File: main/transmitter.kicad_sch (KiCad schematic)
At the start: 35 parts, among them Q1 PZT2222A, Q2 BS170, Q3 BS170, Q4 BS170, Q5 BS170, Q6 MMBT3904, Q7 BSS84, Q8 BS170, Q9 MMBT3904

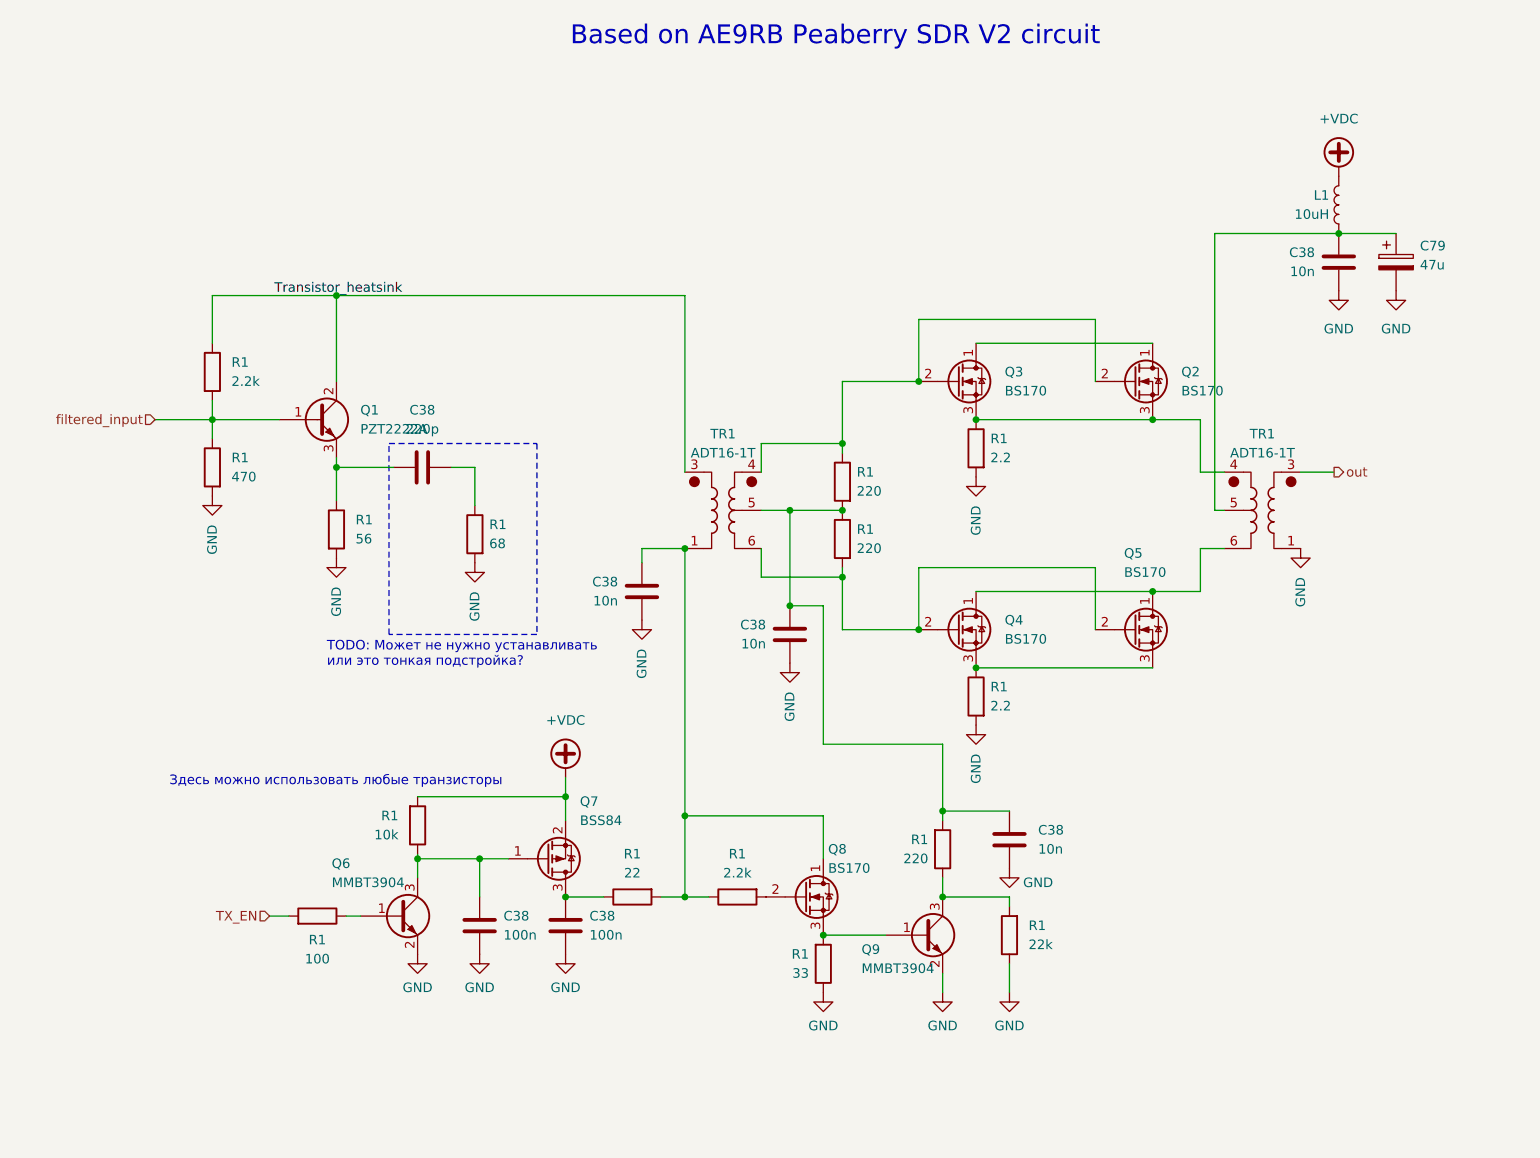
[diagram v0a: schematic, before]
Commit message: Power amplifier redraw
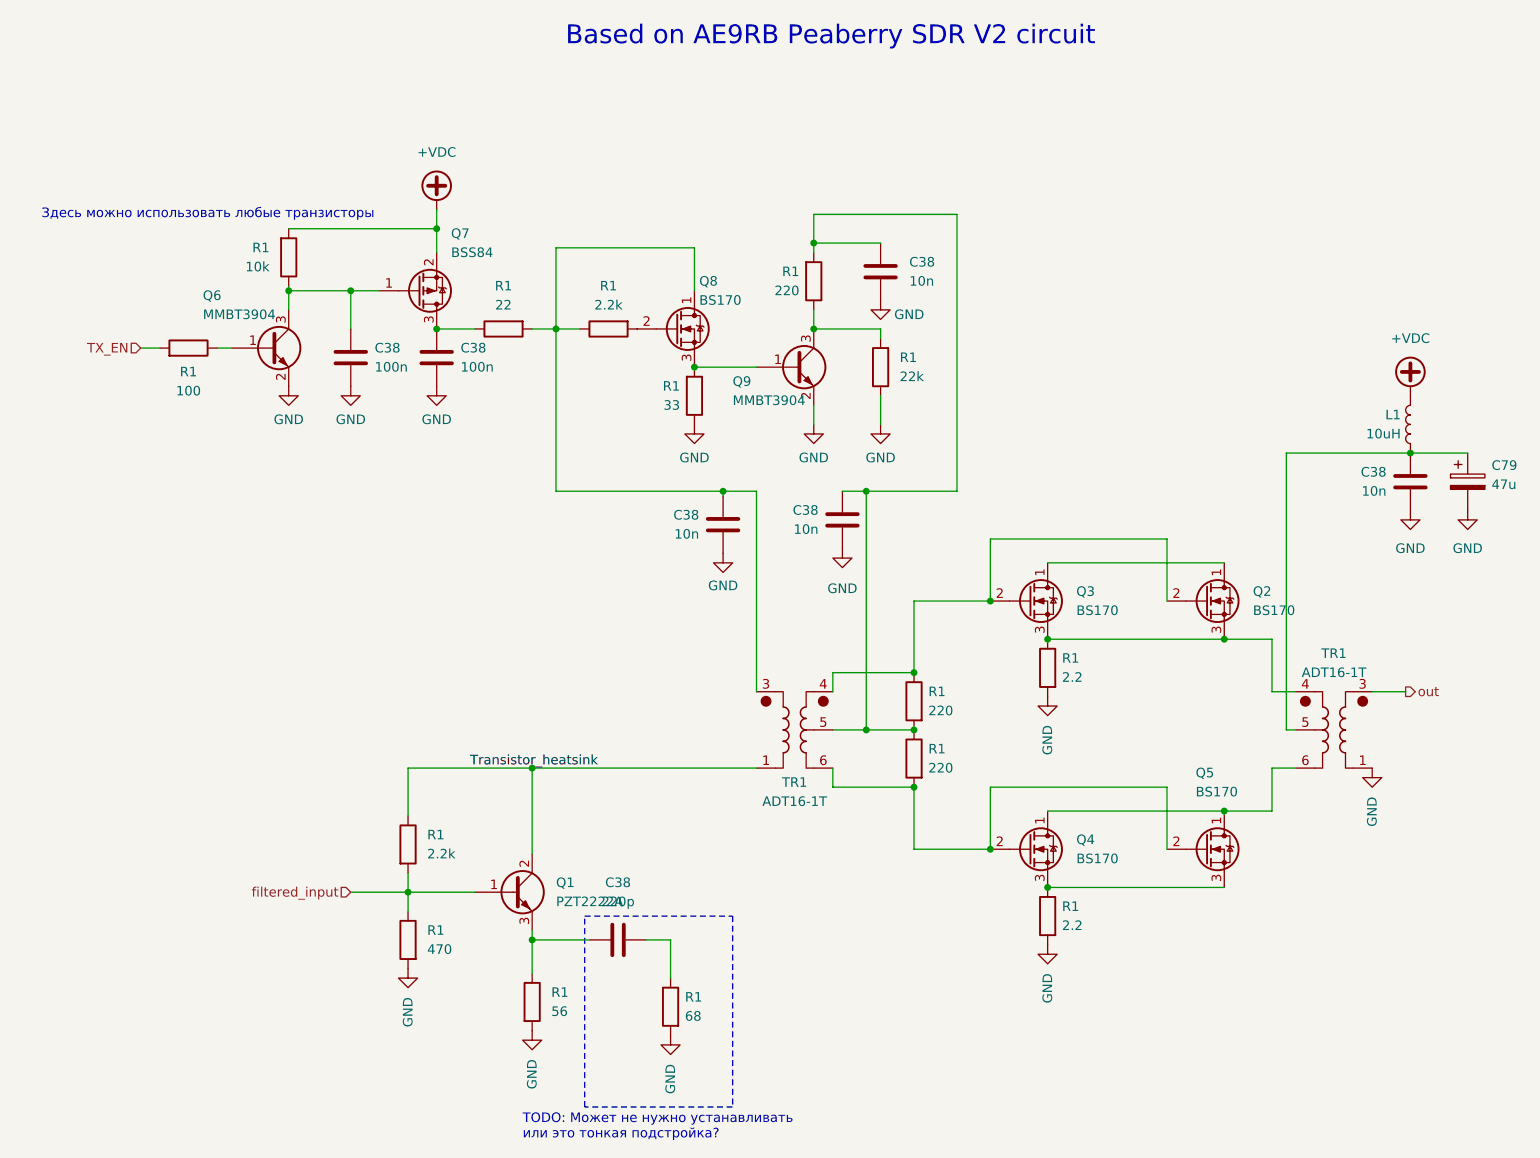
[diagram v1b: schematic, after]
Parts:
- removed C38 (x2): 100n, symbol Device:C
- removed C38: 10n, symbol Device:C
- removed R1: 2.2k, symbol Device:R
- removed R1: 10k, symbol Device:R
- removed R1: 22k, symbol Device:R
- removed R1: 33, symbol Device:R
- removed R1: 100, symbol Device:R
- removed R1: 220, symbol Device:R
- removed R1: 22, symbol Device:R
- added C38 (x2): 100n, symbol Device:C
- added C38: 10n, symbol Device:C
- added R1: 10k, symbol Device:R
- added R1: 33, symbol Device:R
- added R1: 100, symbol Device:R
- added R1: 220, symbol Device:R
- added R1: 22, symbol Device:R
- added R1: 22k, symbol Device:R
- added R1: 2.2k, symbol Device:R
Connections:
- net +VDC: now also R1.2
- net GND: now also C38.1, C38.1, C38.1, R1.1, R1.1
- net TX_EN: now also R1.2
- net Transistor_heatsink: now also TR1.1; no longer TR1.3
- net at C38.2, Q8.1 (D): now also TR1.3, R1.1, R1.2; no longer TR1.1
- net at Q8.2 (G): now also R1.2
- net at Q6.3 (C), Q7.1 (G): now also C38.2, R1.1
- net at Q9.3 (C): now also R1.1, R1.2
- net at Q8.3 (S), Q9.1 (B): now also R1.2
- net at Q6.1 (B): now also R1.1
- net at Q7.3 (D): now also C38.2, R1.1
- net at C38.2, R1.1, R1.2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: now also C38.2, R1.2
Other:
- moved on the sheet: C38, C79, L1, Q1, Q2, Q3, Q4, Q5, R1, TR1

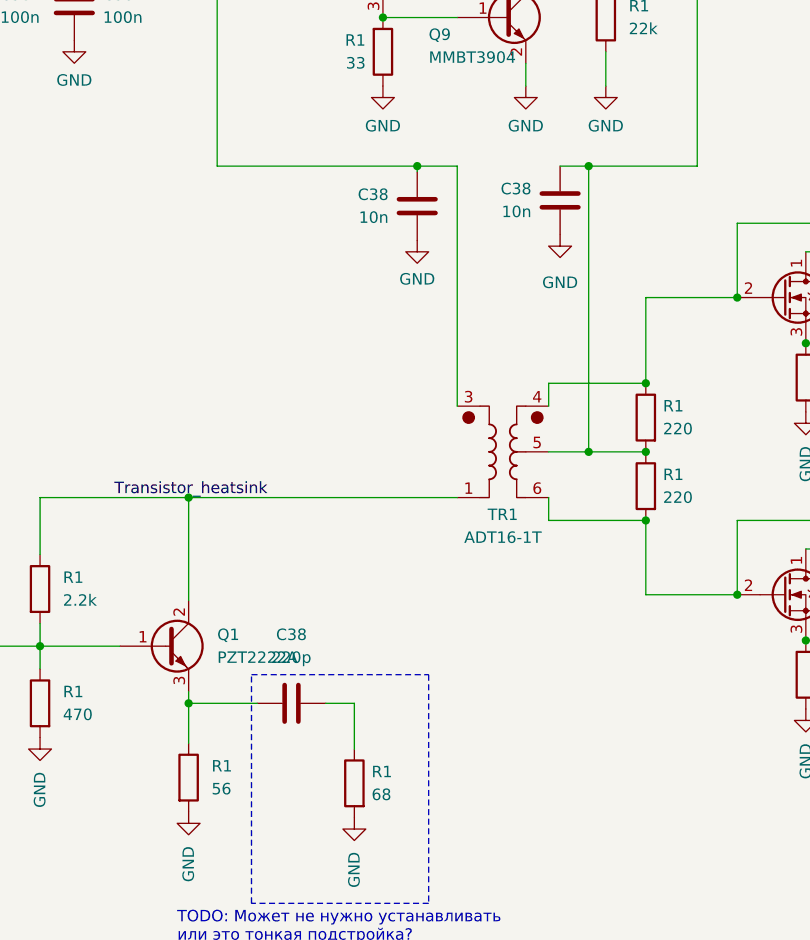
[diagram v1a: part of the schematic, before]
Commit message: 30 MHz output LPF added
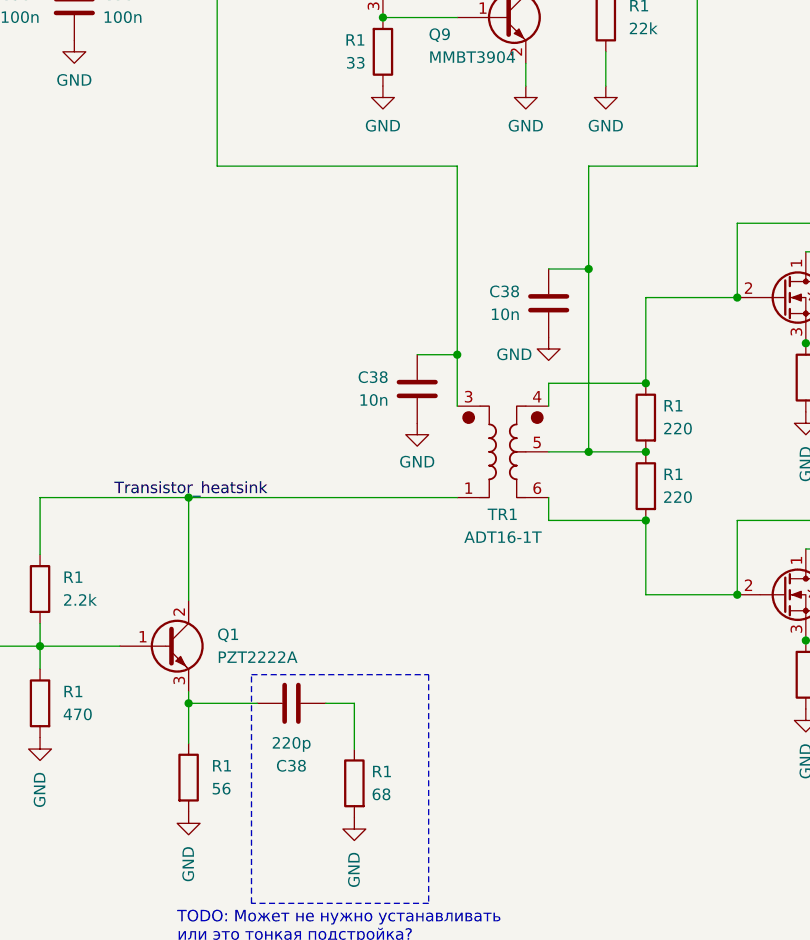
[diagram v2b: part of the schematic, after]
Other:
- moved on the sheet: C38
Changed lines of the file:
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@@
   (junction (at 147.955 112.395) (diameter 0) (color 0 0 0 0)
   )
+  (junction (at 147.955 92.075) (diameter 0) (color 0 0 0 0)
+  )
   (junction (at 90.805 45.72) (diameter 0) (color 0 0 0 0)
   )
@@
   (junction (at 154.305 112.395) (diameter 0) (color 0 0 0 0)
   )
-  (junction (at 147.955 80.645) (diameter 0) (color 0 0 0 0)
-  )
   (junction (at 140.97 47.625) (diameter 0) (color 0 0 0 0)
   )
@@
   (junction (at 172.085 100.33) (diameter 0) (color 0 0 0 0)
   )
-  (junction (at 128.905 80.645) (diameter 0) (color 0 0 0 0)
-  )
   (junction (at 71.12 53.975) (diameter 0) (color 0 0 0 0)
   )
@@
   (junction (at 195.58 100.33) (diameter 0) (color 0 0 0 0)
   )
+  (junction (at 133.35 101.6) (diameter 0) (color 0 0 0 0)
+  )
   (junction (at 164.465 128.27) (diameter 0) (color 0 0 0 0)
   )
@@
     (stroke (width 0) (type default))
   )
+  (wire (pts (xy 147.955 80.645) (xy 147.955 92.075))
+    (stroke (width 0) (type default))
+  )
   (wire (pts (xy 71.12 53.975) (xy 79.375 53.975))
     (stroke (width 0) (type default))
@@
     (stroke (width 0) (type default))
   )
-  (wire (pts (xy 147.955 80.645) (xy 147.955 112.395))
-    (stroke (width 0) (type default))
-  )
   (wire (pts (xy 140.97 56.515) (xy 140.97 59.055))
     (stroke (width 0) (type default))
@@
     (stroke (width 0) (type default))
   )
-  (wire (pts (xy 133.35 80.645) (xy 133.35 107.315))
+  (wire (pts (xy 133.35 80.645) (xy 133.35 101.6))
     (stroke (width 0) (type default))
   )
@@
     (stroke (width 0) (type default))
   )
-  (wire (pts (xy 106.68 80.645) (xy 128.905 80.645))
-    (stroke (width 0) (type default))
-  )
   (wire (pts (xy 51.435 61.595) (xy 53.975 61.595))
     (stroke (width 0) (type default))
@@
     (stroke (width 0) (type default))
   )
-  (wire (pts (xy 128.905 80.645) (xy 133.35 80.645))
+  (wire (pts (xy 106.68 80.645) (xy 133.35 80.645))
     (stroke (width 0) (type default))
   )
@@
     (stroke (width 0) (type default))
   )
-  (wire (pts (xy 144.78 80.645) (xy 147.955 80.645))
+  (wire (pts (xy 143.51 92.075) (xy 147.955 92.075))
     (stroke (width 0) (type default))
   )
@@
     (stroke (width 0) (type default))
   )
-  (wire (pts (xy 128.905 81.28) (xy 128.905 80.645))
+  (wire (pts (xy 133.35 101.6) (xy 133.35 107.315))
     (stroke (width 0) (type default))
   )
@@
     (stroke (width 0) (type default))
   )
+  (wire (pts (xy 147.955 92.075) (xy 147.955 112.395))
+    (stroke (width 0) (type default))
+  )
   (wire (pts (xy 201.93 123.19) (xy 195.58 123.19))
     (stroke (width 0) (type default))
@@
   )
   (wire (pts (xy 86.995 131.445) (xy 86.995 133.985))
+    (stroke (width 0) (type default))
+  )
+  (wire (pts (xy 128.905 101.6) (xy 133.35 101.6))
     (stroke (width 0) (type default))
   )
@@
     (effects (font (size 1.27 1.27)) (justify right))
   )
-  (symbol (lib_id "Device:C") (at 114.935 140.335 90) (mirror x) (unit 1)
-    (in_bom yes) (on_board yes) (dnp no) (fields_autoplaced)
-    (property "Reference" "C38" (at 114.935 132.715 90)
-      (effects (font (size 1.27 1.27)))
-    )
-    (property "Value" "220p" (at 114.935 135.255 90)
-      (effects (font (size 1.27 1.27)))
-    )
-    (property "Footprint" "" (at 118.745 141.3002 0)
+  (symbol (lib_id "Device:C") (at 114.935 140.335 90) (unit 1)
+    (in_bom yes) (on_board yes) (dnp no)
+    (property "Reference" "C38" (at 114.935 147.32 90)
+      (effects (font (size 1.27 1.27)))
+    )
+    (property "Value" "220p" (at 114.935 144.78 90)
+      (effects (font (size 1.27 1.27)))
+    )
+    (property "Footprint" "" (at 118.745 139.3698 0)
       (effects (font (size 1.27 1.27)) hide)
     )
@@
     )
   )
-  (symbol (lib_id "Device:C") (at 128.905 85.09 0) (mirror x) (unit 1)
-    (in_bom yes) (on_board yes) (dnp no) (fields_autoplaced)
-    (property "Reference" "C38" (at 125.73 83.82 0)
-      (effects (font (size 1.27 1.27)) (justify right))
-    )
-    (property "Value" "10n" (at 125.73 86.36 0)
-      (effects (font (size 1.27 1.27)) (justify right))
-    )
-    (property "Footprint" "" (at 129.8702 81.28 0)
-      (effects (font (size 1.27 1.27)) hide)
-    )
-    (property "Datasheet" "~" (at 128.905 85.09 0)
+  (symbol (lib_id "Device:C") (at 128.905 105.41 0) (mirror x) (unit 1)
+    (in_bom yes) (on_board yes) (dnp no) (fields_autoplaced)
+    (property "Reference" "C38" (at 125.73 104.14 0)
+      (effects (font (size 1.27 1.27)) (justify right))
+    )
+    (property "Value" "10n" (at 125.73 106.68 0)
+      (effects (font (size 1.27 1.27)) (justify right))
+    )
+    (property "Footprint" "" (at 129.8702 101.6 0)
+      (effects (font (size 1.27 1.27)) hide)
+    )
+    (property "Datasheet" "~" (at 128.905 105.41 0)
       (effects (font (size 1.27 1.27)) hide)
     )
@@
     )
   )
-  (symbol (lib_id "Device:C") (at 144.78 84.455 0) (mirror x) (unit 1)
-    (in_bom yes) (on_board yes) (dnp no) (fields_autoplaced)
-    (property "Reference" "C38" (at 141.605 83.185 0)
-      (effects (font (size 1.27 1.27)) (justify right))
-    )
-    (property "Value" "10n" (at 141.605 85.725 0)
-      (effects (font (size 1.27 1.27)) (justify right))
-    )
-    (property "Footprint" "" (at 145.7452 80.645 0)
-      (effects (font (size 1.27 1.27)) hide)
-    )
-    (property "Datasheet" "~" (at 144.78 84.455 0)
+  (symbol (lib_id "Device:C") (at 143.51 95.885 0) (mirror x) (unit 1)
+    (in_bom yes) (on_board yes) (dnp no) (fields_autoplaced)
+    (property "Reference" "C38" (at 140.335 94.615 0)
+      (effects (font (size 1.27 1.27)) (justify right))
+    )
+    (property "Value" "10n" (at 140.335 97.155 0)
+      (effects (font (size 1.27 1.27)) (justify right))
+    )
+    (property "Footprint" "" (at 144.4752 92.075 0)
+      (effects (font (size 1.27 1.27)) hide)
+    )
+    (property "Datasheet" "~" (at 143.51 95.885 0)
       (effects (font (size 1.27 1.27)) hide)
     )
@@
     )
   )
-  (symbol (lib_id "power:GND") (at 144.78 88.265 0) (mirror y) (unit 1)
-    (in_bom yes) (on_board yes) (dnp no) (fields_autoplaced)
-    (property "Reference" "#PWR022" (at 144.78 94.615 0)
-      (effects (font (size 1.27 1.27)) hide)
-    )
-    (property "Value" "GND" (at 144.78 93.599 0)
-      (effects (font (size 1.27 1.27)))
-    )
-    (property "Footprint" "" (at 144.78 88.265 0)
-      (effects (font (size 1.27 1.27)) hide)
-    )
-    (property "Datasheet" "" (at 144.78 88.265 0)
+  (symbol (lib_id "power:GND") (at 143.51 99.695 0) (mirror y) (unit 1)
+    (in_bom yes) (on_board yes) (dnp no) (fields_autoplaced)
+    (property "Reference" "#PWR022" (at 143.51 106.045 0)
+      (effects (font (size 1.27 1.27)) hide)
+    )
+    (property "Value" "GND" (at 139.7 101.6 0)
+      (effects (font (size 1.27 1.27)))
+    )
+    (property "Footprint" "" (at 143.51 99.695 0)
+      (effects (font (size 1.27 1.27)) hide)
+    )
+    (property "Datasheet" "" (at 143.51 99.695 0)
       (effects (font (size 1.27 1.27)) hide)
     )
@@
     )
   )
-  (symbol (lib_id "power:GND") (at 128.905 88.9 0) (mirror y) (unit 1)
-    (in_bom yes) (on_board yes) (dnp no) (fields_autoplaced)
-    (property "Reference" "#PWR022" (at 128.905 95.25 0)
-      (effects (font (size 1.27 1.27)) hide)
-    )
-    (property "Value" "GND" (at 128.905 93.218 0)
-      (effects (font (size 1.27 1.27)))
-    )
-    (property "Footprint" "" (at 128.905 88.9 0)
-      (effects (font (size 1.27 1.27)) hide)
-    )
-    (property "Datasheet" "" (at 128.905 88.9 0)
-      (effects (font (size 1.27 1.27)) hide)
-    )
+  (symbol (lib_id "power:GND") (at 128.905 109.22 0) (mirror y) (unit 1)
+    (in_bom yes) (on_board yes) (dnp no) (fields_autoplaced)
+    (property "Reference" "#PWR022" (at 128.905 115.57 0)
+      (effects (font (size 1.27 1.27)) hide)
+    )
+    (property "Value" "GND" (at 128.905 113.538 0)
+      (effects (font (size 1.27 1.27)))
+    )
+    (property "Footprint" "" (at 128.905 109.22 0)
+      (effects (font (size 1.27 1.27)) hide)
+    )
+    (property "Datasheet" "" (at 128.905 109.22 0)
+      (effects (font (size 1.27 1.27)) hide)
+    )
